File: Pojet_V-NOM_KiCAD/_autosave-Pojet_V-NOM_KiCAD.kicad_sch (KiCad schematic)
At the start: 0 parts

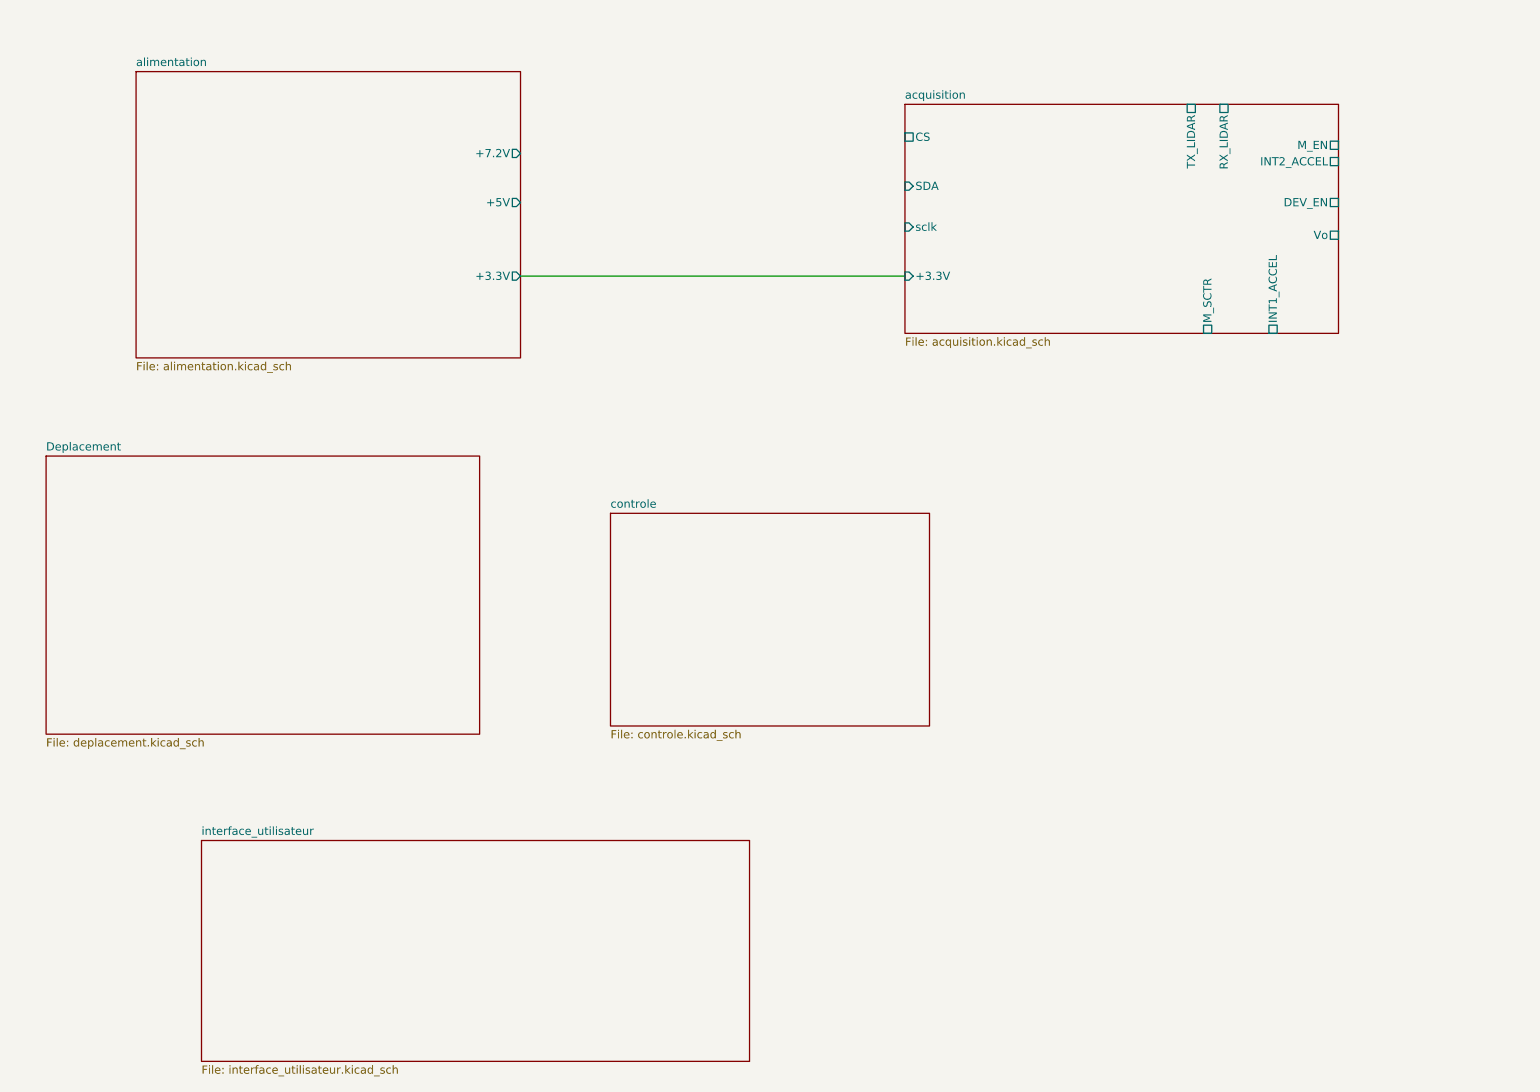
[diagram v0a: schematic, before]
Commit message: modif
modif
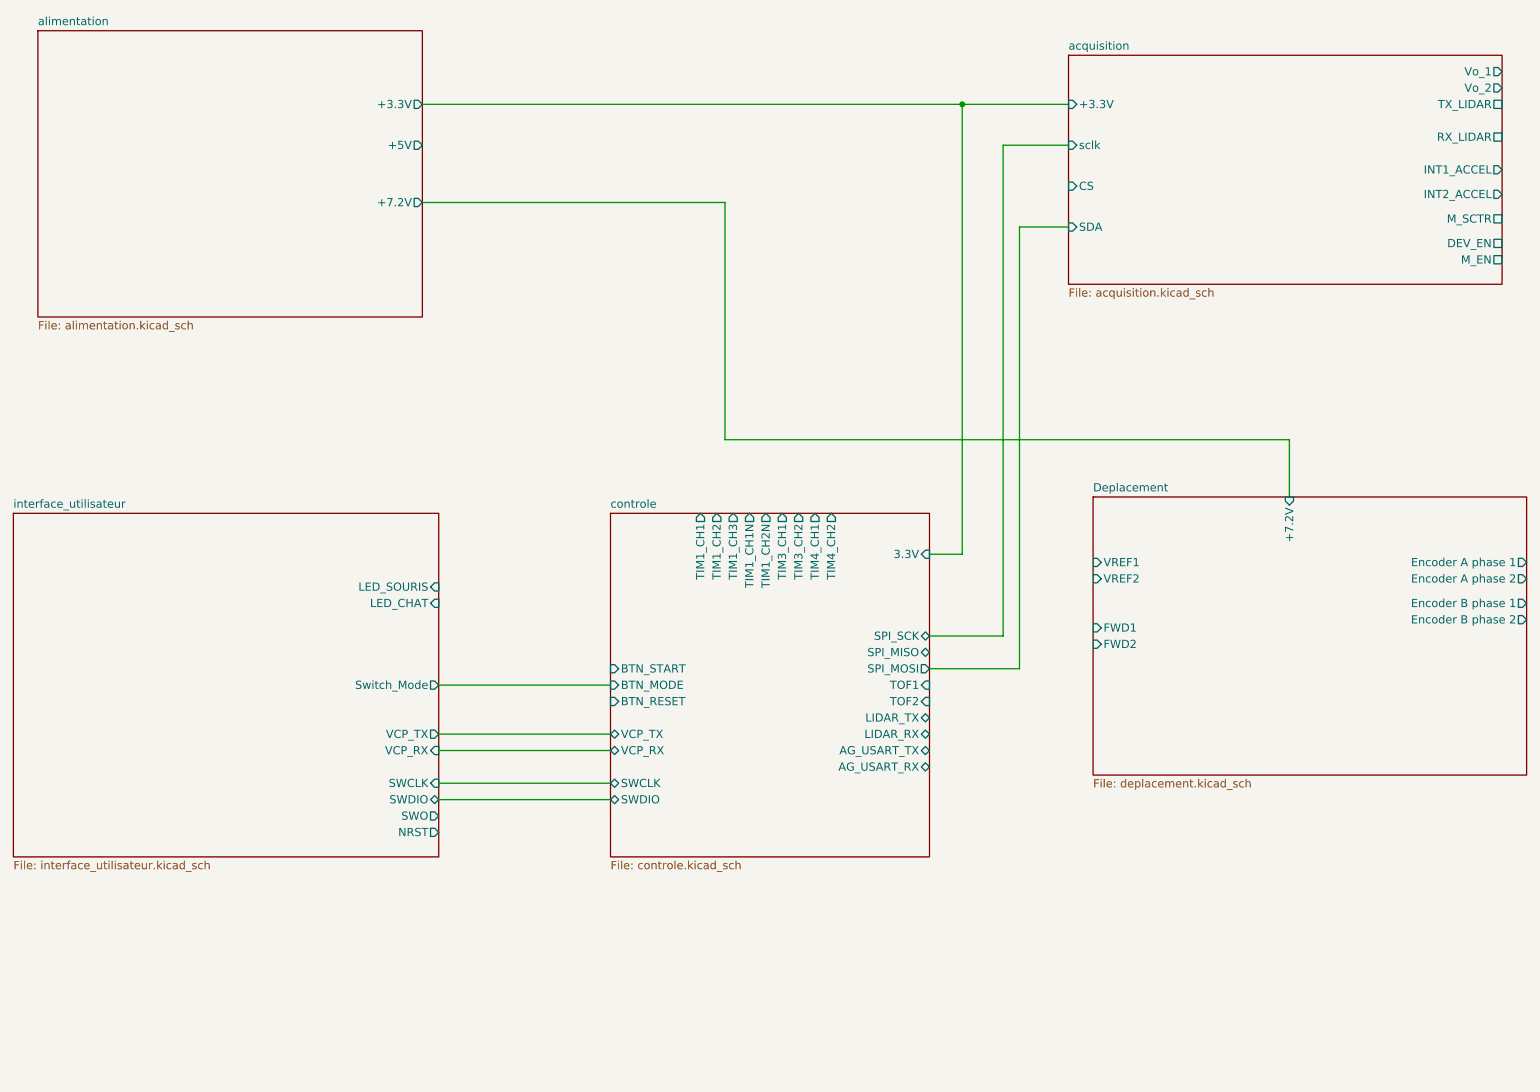
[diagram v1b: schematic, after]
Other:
- sheet Deplacement ports: added +7.2V, Encoder A phase 1, Encoder A phase 2, Encoder B phase 1, Encoder B phase 2, FWD1, FWD2, VREF1, VREF2; removed none
- sheet acquisition ports: added Vo_1, Vo_2; removed Vo
- sheet controle ports: added 3.3V, AG_USART_RX, AG_USART_TX, BTN_MODE, BTN_RESET, BTN_START, LIDAR_RX, LIDAR_TX, SPI_MISO, SPI_MOSI, SPI_SCK, SWCLK, SWDIO, TIM1_CH1, TIM1_CH1N, TIM1_CH2, TIM1_CH2N, TIM1_CH3, TIM3_CH1, TIM3_CH2, TIM4_CH1, TIM4_CH2, TOF1, TOF2, VCP_RX, VCP_TX; removed none
- sheet interface_utilisateur ports: added LED_CHAT, LED_SOURIS, NRST, SWCLK, SWDIO, SWO, Switch_Mode, VCP_RX, VCP_TX; removed none
